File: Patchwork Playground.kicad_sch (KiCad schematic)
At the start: 93 parts, among them J1 PADS, J2 USB_C_Receptacle_USB2.0, J3 PADS, J4 POGO, J5 PADS, J6 JST-GH-4P, SW1 SW_SPDT, SW2 SW_SPDT, SW3 SW_SPDT, SW4 BUTTON, SW5 SW_SPDT, SW6 SW_SPDT, SW7 SW_SPDT, U1 SMF05CT1G, U2 M3406, U3 BQ21040DBVR, U4 SMF05CT1G, U5 QMC5883L, U6 BC805M, U7 LSM6DSV

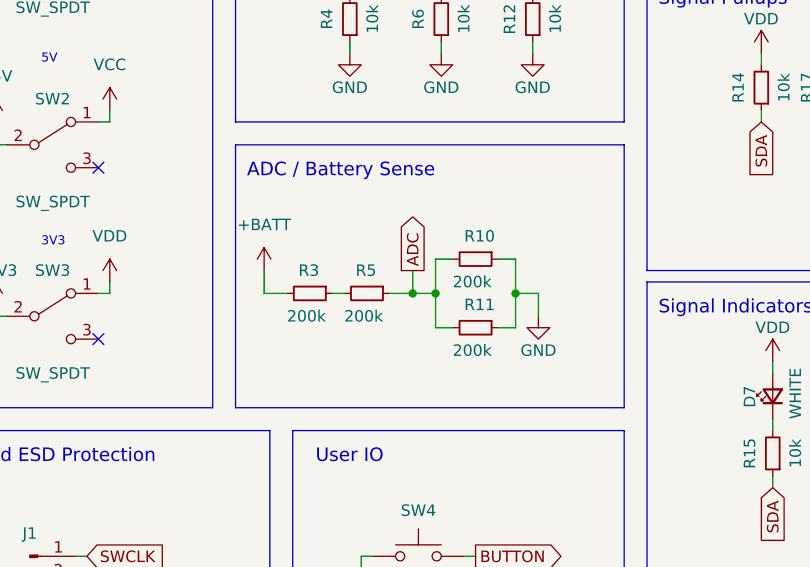
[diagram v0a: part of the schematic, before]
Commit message: update board img
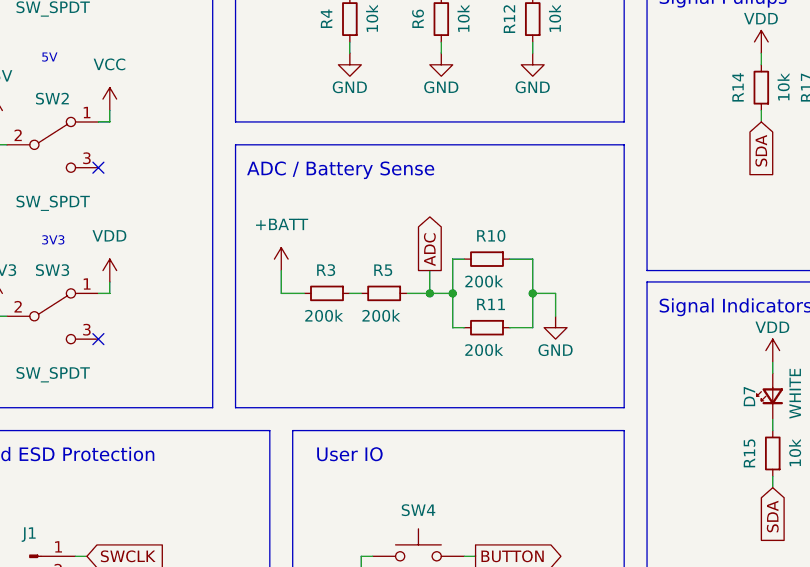
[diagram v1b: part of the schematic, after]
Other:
- moved on the sheet: R10, R11, R3, R5
